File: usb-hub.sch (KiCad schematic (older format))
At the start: 45 parts, among them J1 USB_C_Receptacle_16pin, J2 USB_C_Receptacle_16pin, J3 USB_C_Receptacle_16pin, P1 CONN_02X03, Q1 Q_PMOS_GSD 2A, Q2 Q_NMOS_GSD 1Amp, SW1 SW_Push, U1 usblc6-4, U2 LY2508, U3 samd21g, U4 4 pin RGB led, com anode, red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, Y1 32.768khz

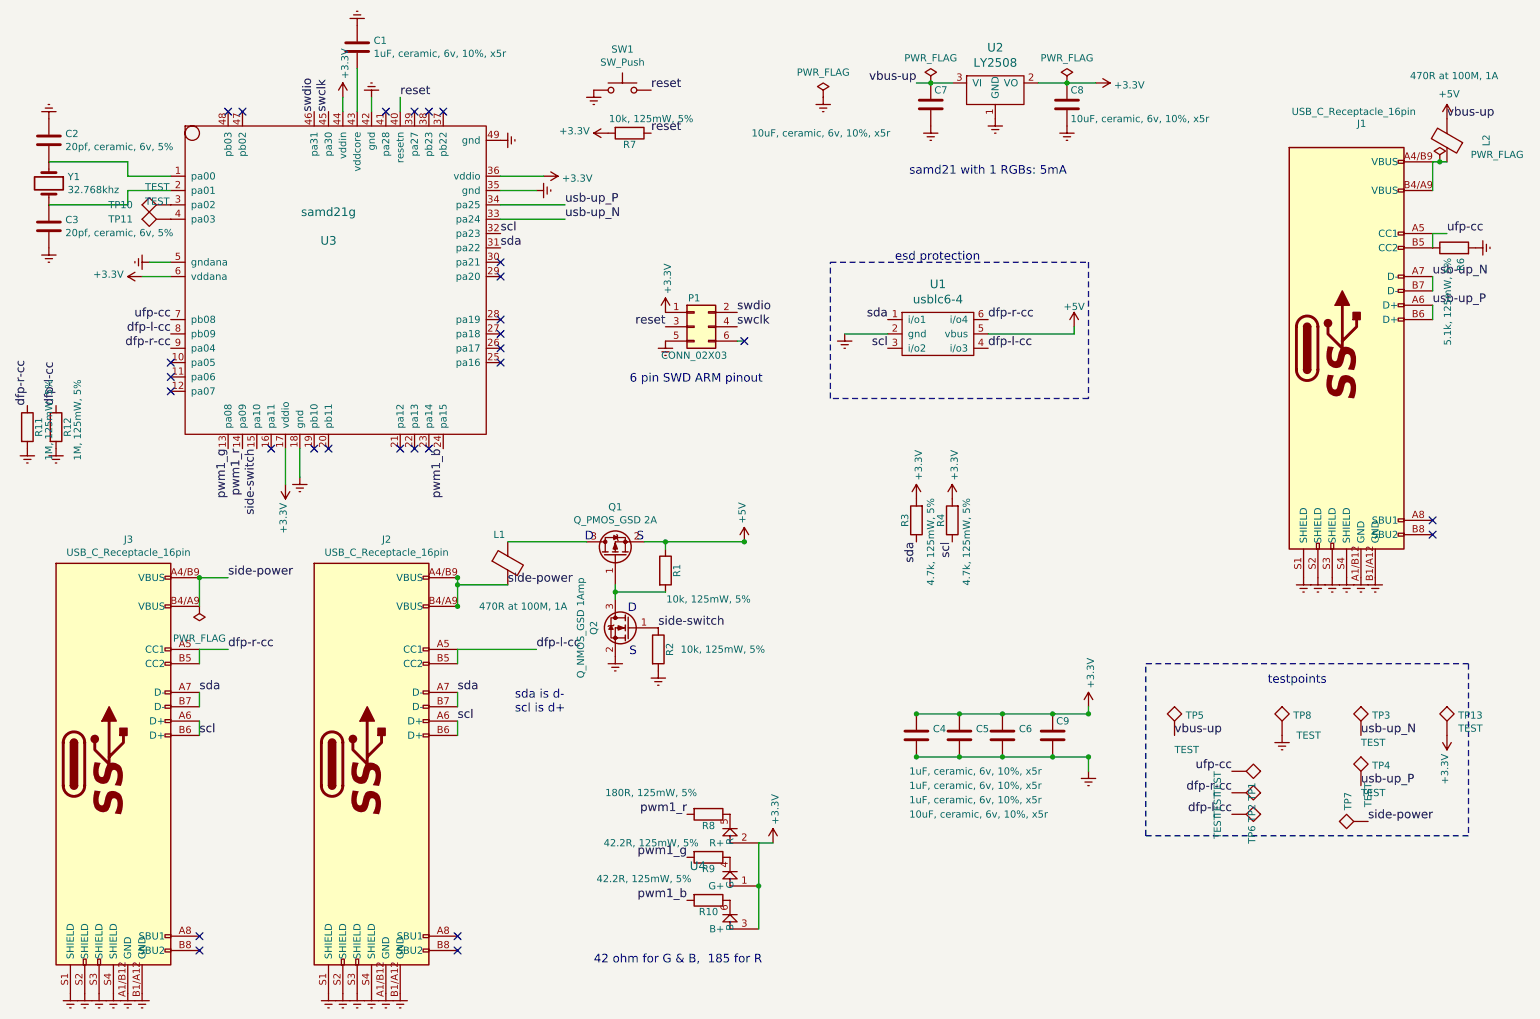
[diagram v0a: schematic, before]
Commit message: added holes
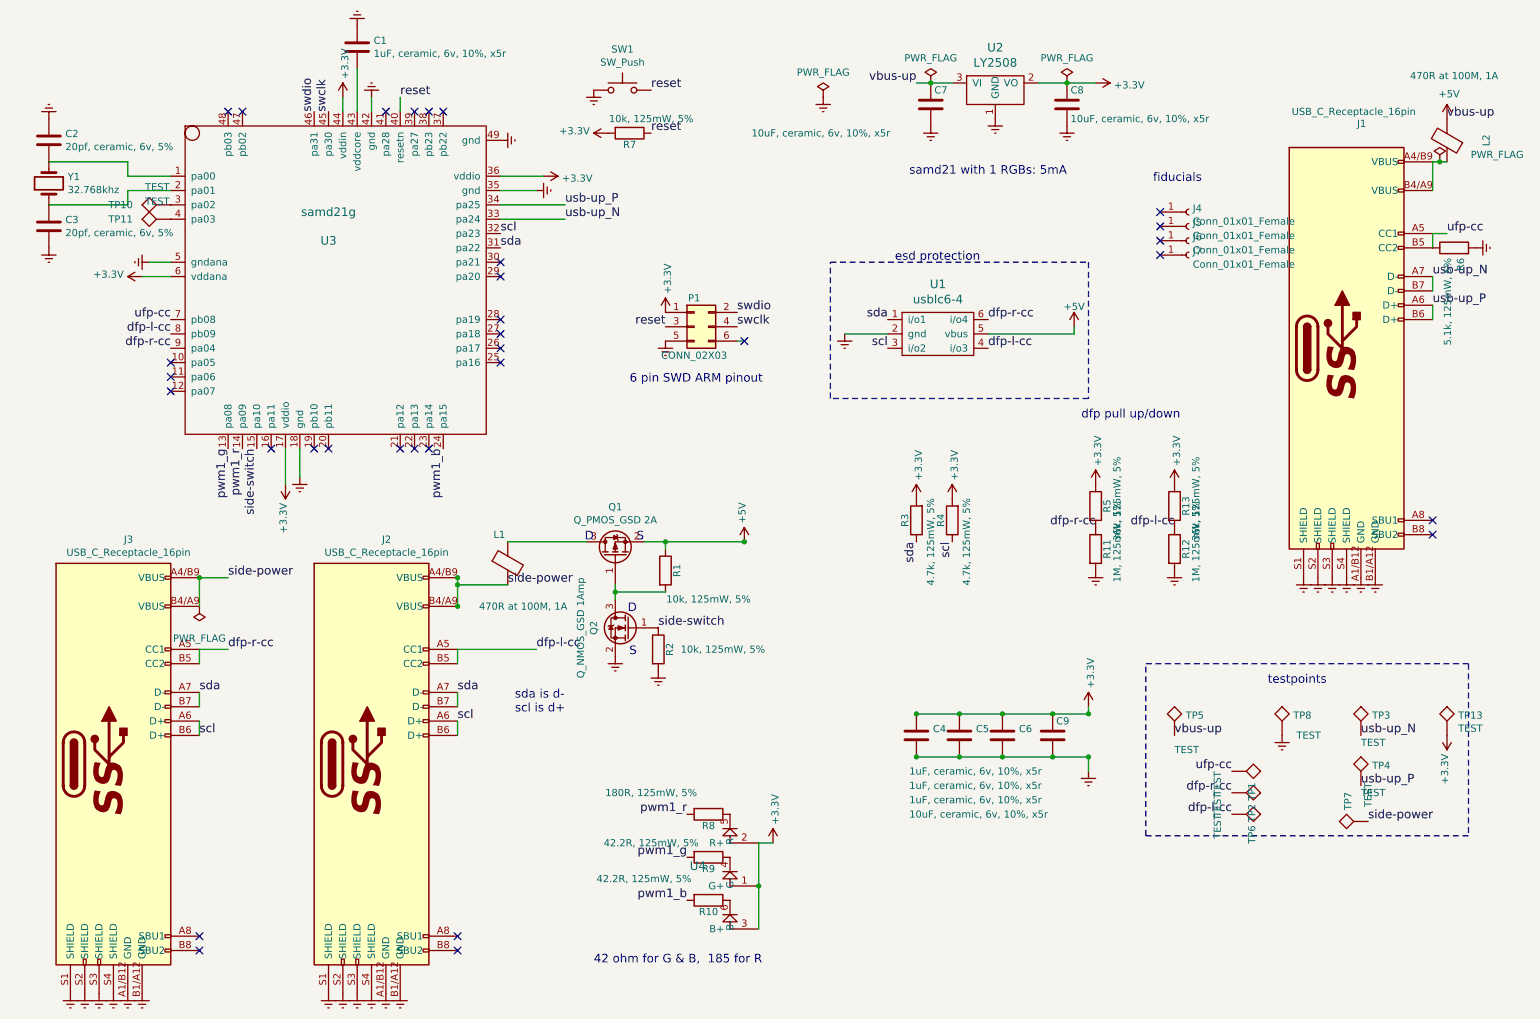
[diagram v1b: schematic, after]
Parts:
- added J4, J5, J6, J7: Conn_01x01_Female, raise_fp:Fiducial_0.5mm_Dia_1mm_Outer, symbol Conn_01x01_Female
- added R13, R5: 36k, 125mW, 5%, raise_fp:R_0603, symbol R
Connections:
- net +3V3: now also R13.1, R5.1
- net dfp-l-cc: now also R13.2
- net dfp-r-cc: now also R5.2
- no-connect marks 28 -> 32
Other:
- note added: "dfp pull up/down"
- note added: "fiducials"
- moved on the sheet: R11, R12
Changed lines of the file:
@@
 L R R11
 U 1 1 5B164F68
-P 750 3550
-F 0 "R11" V 830 3550 50  0000 C CNN
-F 1 "1M, 125mW, 5%" V 900 3600 50  0000 C CNN
-F 2 "raise_fp:R_0603" V 680 3550 30  0001 C CNN
-F 3 "" H 750 3550 30  0000 C CNN
-F 4 "2073351" H 750 3550 60  0001 C CNN "farnell #"
-F 5 "any/open" H -3750 50  60  0001 C CNN "supplier"
-F 6 "Value" H 750 3550 60  0001 C CNN "supplier PN"
-F 7 "Value" H 750 3550 60  0001 C CNN "MOQ"
-F 8 "Value" H 750 3550 60  0001 C CNN "leadtime"
-	1    750  3550
+P 8200 4400
+F 0 "R11" V 8280 4400 50  0000 C CNN
+F 1 "1M, 125mW, 5%" V 8350 4450 50  0000 C CNN
+F 2 "raise_fp:R_0603" V 8130 4400 30  0001 C CNN
+F 3 "" H 8200 4400 30  0000 C CNN
+F 4 "2073351" H 8200 4400 60  0001 C CNN "farnell #"
+F 5 "any/open" H 3700 900 60  0001 C CNN "supplier"
+F 6 "Value" H 8200 4400 60  0001 C CNN "supplier PN"
+F 7 "Value" H 8200 4400 60  0001 C CNN "MOQ"
+F 8 "Value" H 8200 4400 60  0001 C CNN "leadtime"
+	1    8200 4400
 	1    0    0    -1
 $EndComp
@@
 L Earth #PWR049
 U 1 1 5B1650D8
-P 750 3700
-F 0 "#PWR049" H 750 3450 50  0001 C CNN
-F 1 "Earth" H 750 3550 50  0001 C CNN
-F 2 "" H 750 3700 60  0000 C CNN
-F 3 "" H 750 3700 60  0000 C CNN
-	1    750  3700
+P 8200 4550
+F 0 "#PWR049" H 8200 4300 50  0001 C CNN
+F 1 "Earth" H 8200 4400 50  0001 C CNN
+F 2 "" H 8200 4550 60  0000 C CNN
+F 3 "" H 8200 4550 60  0000 C CNN
+	1    8200 4550
 	1    0    0    -1
 $EndComp
@@
 L Earth #PWR052
 U 1 1 5B165141
-P 950 3700
-F 0 "#PWR052" H 950 3450 50  0001 C CNN
-F 1 "Earth" H 950 3550 50  0001 C CNN
-F 2 "" H 950 3700 60  0000 C CNN
-F 3 "" H 950 3700 60  0000 C CNN
-	1    950  3700
+P 8750 4550
+F 0 "#PWR052" H 8750 4300 50  0001 C CNN
+F 1 "Earth" H 8750 4400 50  0001 C CNN
+F 2 "" H 8750 4550 60  0000 C CNN
+F 3 "" H 8750 4550 60  0000 C CNN
+	1    8750 4550
 	1    0    0    -1
 $EndComp
@@
 L R R12
 U 1 1 5B165592
-P 950 3550
-F 0 "R12" V 1030 3550 50  0000 C CNN
-F 1 "1M, 125mW, 5%" V 1100 3600 50  0000 C CNN
-F 2 "raise_fp:R_0603" V 880 3550 30  0001 C CNN
-F 3 "" H 950 3550 30  0000 C CNN
-F 4 "2073351" H 950 3550 60  0001 C CNN "farnell #"
-F 5 "any/open" H -3550 50  60  0001 C CNN "supplier"
-F 6 "Value" H 950 3550 60  0001 C CNN "supplier PN"
-F 7 "Value" H 950 3550 60  0001 C CNN "MOQ"
-F 8 "Value" H 950 3550 60  0001 C CNN "leadtime"
-	1    950  3550
-	1    0    0    -1
-$EndComp
-Text Label 750  3400 1    60   ~ 0
+P 8750 4400
+F 0 "R12" V 8830 4400 50  0000 C CNN
+F 1 "1M, 125mW, 5%" V 8900 4450 50  0000 C CNN
+F 2 "raise_fp:R_0603" V 8680 4400 30  0001 C CNN
+F 3 "" H 8750 4400 30  0000 C CNN
+F 4 "2073351" H 8750 4400 60  0001 C CNN "farnell #"
+F 5 "any/open" H 4250 900 60  0001 C CNN "supplier"
+F 6 "Value" H 8750 4400 60  0001 C CNN "supplier PN"
+F 7 "Value" H 8750 4400 60  0001 C CNN "MOQ"
+F 8 "Value" H 8750 4400 60  0001 C CNN "leadtime"
+	1    8750 4400
+	1    0    0    -1
+$EndComp
+Text Label 8200 4250 2    60   ~ 0
 dfp-r-cc
-Text Label 950  3400 1    60   ~ 0
+Text Label 8750 4250 2    60   ~ 0
 dfp-l-cc
 Text Notes 4950 3250 0    60   ~ 0
@@
 Text Label 7200 4350 3    60   ~ 0
 scl
+$Comp
+L R R5
+U 1 1 5B30E926
+P 8200 4100
+F 0 "R5" V 8280 4100 50  0000 C CNN
+F 1 "36k, 125mW, 5%" V 8350 4150 50  0000 C CNN
+F 2 "raise_fp:R_0603" V 8130 4100 30  0001 C CNN
+F 3 "" H 8200 4100 30  0000 C CNN
+F 4 "2447349" H 8200 4100 60  0001 C CNN "farnell #"
+F 5 "any/open" H 3700 600 60  0001 C CNN "supplier"
+F 6 "Value" H 8200 4100 60  0001 C CNN "supplier PN"
+F 7 "Value" H 8200 4100 60  0001 C CNN "MOQ"
+F 8 "Value" H 8200 4100 60  0001 C CNN "leadtime"
+	1    8200 4100
+	1    0    0    -1
+$EndComp
+$Comp
+L R R13
+U 1 1 5B30E9DE
+P 8750 4100
+F 0 "R13" V 8830 4100 50  0000 C CNN
+F 1 "36k, 125mW, 5%" V 8900 4150 50  0000 C CNN
+F 2 "raise_fp:R_0603" V 8680 4100 30  0001 C CNN
+F 3 "" H 8750 4100 30  0000 C CNN
+F 4 "2447349" H 8750 4100 60  0001 C CNN "farnell #"
+F 5 "any/open" H 4250 600 60  0001 C CNN "supplier"
+F 6 "Value" H 8750 4100 60  0001 C CNN "supplier PN"
+F 7 "Value" H 8750 4100 60  0001 C CNN "MOQ"
+F 8 "Value" H 8750 4100 60  0001 C CNN "leadtime"
+	1    8750 4100
+	1    0    0    -1
+$EndComp
+$Comp
+L +3.3V #PWR026
+U 1 1 5B30ED4A
+P 8750 3950
+F 0 "#PWR026" H 8750 3800 50  0001 C CNN
+F 1 "+3.3V" V 8765 4078 50  0000 L CNN
+F 2 "" H 8750 3950 50  0001 C CNN
+F 3 "" H 8750 3950 50  0001 C CNN
+	1    8750 3950
+	1    0    0    -1
+$EndComp
+$Comp
+L +3.3V #PWR027
+U 1 1 5B30EDE2
+P 8200 3950
+F 0 "#PWR027" H 8200 3800 50  0001 C CNN
+F 1 "+3.3V" V 8215 4078 50  0000 L CNN
+F 2 "" H 8200 3950 50  0001 C CNN
+F 3 "" H 8200 3950 50  0001 C CNN
+	1    8200 3950
+	1    0    0    -1
+$EndComp
+Text Notes 8100 3500 0    60   ~ 0
+dfp pull up/down
+$Comp
+L Conn_01x01_Female J5
+U 1 1 5B310461
+P 8850 2150
+F 0 "J5" H 8877 2176 50  0000 L CNN
+F 1 "Conn_01x01_Female" H 8877 2085 50  0000 L CNN
+F 2 "raise_fp:Fiducial_0.5mm_Dia_1mm_Outer" H 8850 2150 50  0001 C CNN
+F 3 "~" H 8850 2150 50  0001 C CNN
+	1    8850 2150
+	1    0    0    -1
+$EndComp
+NoConn ~ 8650 2150
+$Comp
+L Conn_01x01_Female J4
+U 1 1 5B310711
+P 8850 2050
+F 0 "J4" H 8877 2076 50  0000 L CNN
+F 1 "Conn_01x01_Female" H 8877 1985 50  0000 L CNN
+F 2 "raise_fp:Fiducial_0.5mm_Dia_1mm_Outer" H 8850 2050 50  0001 C CNN
+F 3 "~" H 8850 2050 50  0001 C CNN
+	1    8850 2050
+	1    0    0    -1
+$EndComp
+NoConn ~ 8650 2050
+$Comp
+L Conn_01x01_Female J7
+U 1 1 5B3107E3
+P 8850 2350
+F 0 "J7" H 8877 2376 50  0000 L CNN
+F 1 "Conn_01x01_Female" H 8877 2285 50  0000 L CNN
+F 2 "raise_fp:Fiducial_0.5mm_Dia_1mm_Outer" H 8850 2350 50  0001 C CNN
+F 3 "~" H 8850 2350 50  0001 C CNN
+	1    8850 2350
+	1    0    0    -1
+$EndComp
+NoConn ~ 8650 2350
+$Comp
+L Conn_01x01_Female J6
+U 1 1 5B3107EA
+P 8850 2250
+F 0 "J6" H 8877 2276 50  0000 L CNN
+F 1 "Conn_01x01_Female" H 8877 2185 50  0000 L CNN
+F 2 "raise_fp:Fiducial_0.5mm_Dia_1mm_Outer" H 8850 2250 50  0001 C CNN
+F 3 "~" H 8850 2250 50  0001 C CNN
+	1    8850 2250
+	1    0    0    -1
+$EndComp
+NoConn ~ 8650 2250
+Text Notes 8600 1850 0    60   ~ 0
+fiducials
 $EndSCHEMATC
